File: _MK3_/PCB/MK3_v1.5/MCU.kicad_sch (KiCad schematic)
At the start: 18 parts, among them J11 USB_TypeC, SW1 SW_Push, SW2 SW_Push, SW4 SW_Push, SW5 SW_Push, U1 ESP32-S3-WROOM-1, U3 USBLC6-2SC6

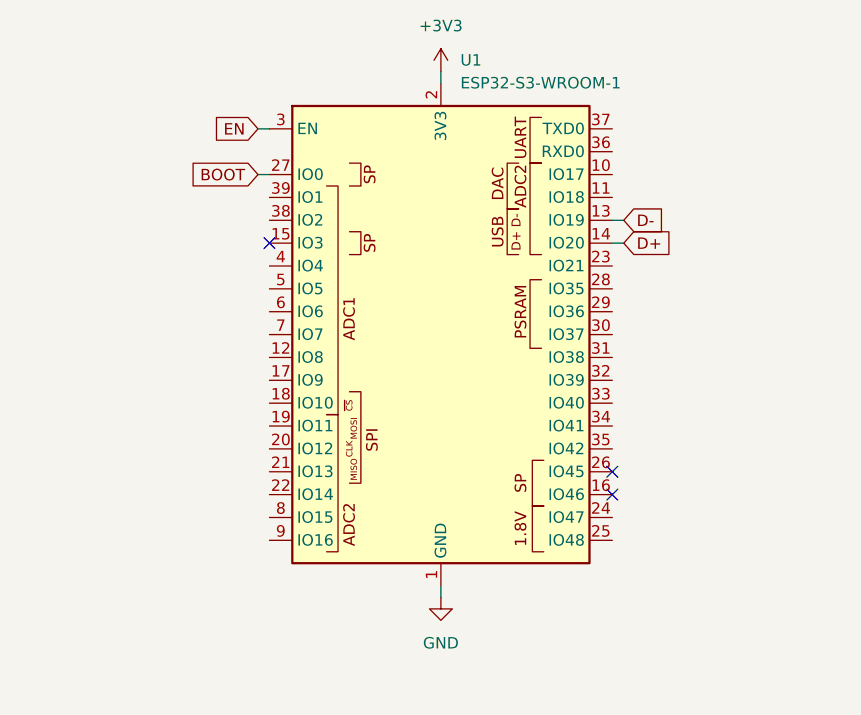
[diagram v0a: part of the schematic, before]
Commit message: pcb done
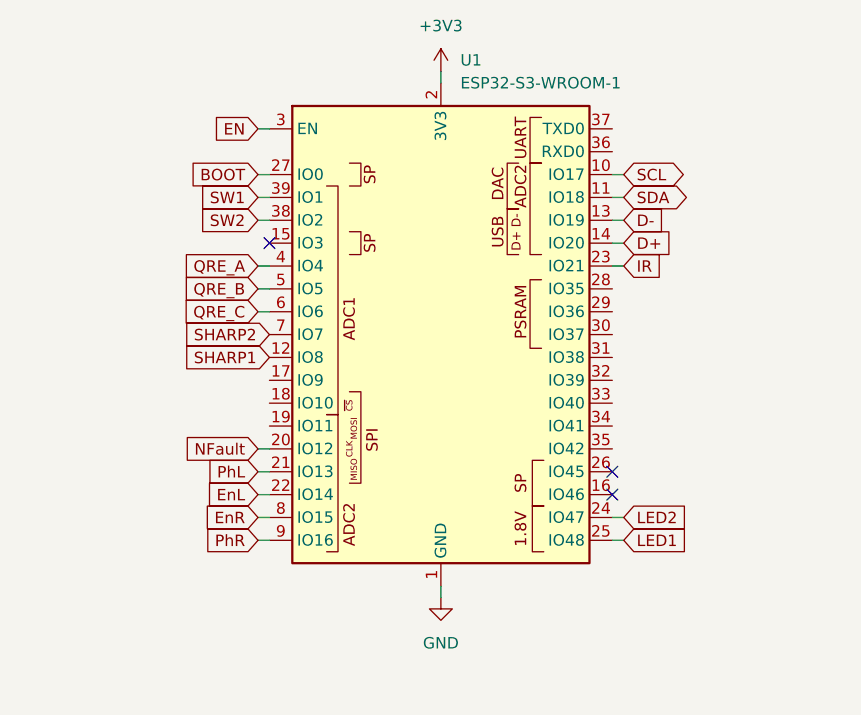
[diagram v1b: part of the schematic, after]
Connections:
- net SW1: now also U1.39 (IO1)
- net SW2: now also U1.38 (IO2)
- net SCL: now reaches U1.10 (IO17)
- net SDA: now reaches U1.11 (IO18)
- net SHARP1: now reaches U1.12 (IO8)
- net NFault: now reaches U1.20 (IO12)
- net PhL: now reaches U1.21 (IO13)
- net EnL: now reaches U1.22 (IO14)
- net IR: now reaches U1.23 (IO21)
- net LED2: now reaches U1.24 (IO47)
- net LED1: now reaches U1.25 (IO48)
- net QRE_A: now reaches U1.4 (IO4)
- net QRE_B: now reaches U1.5 (IO5)
- net QRE_C: now reaches U1.6 (IO6)
- net SHARP2: now reaches U1.7 (IO7)
- net EnR: now reaches U1.8 (IO15)
- net PhR: now reaches U1.9 (IO16)
